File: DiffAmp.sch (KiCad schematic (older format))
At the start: 34 parts, among them J1 USB_OTG, J2 Screw_Terminal_1x03, J3 Conn_01x02, J4 Conn_01x02, J5 Conn_01x02, U1 SF_IHXXXXS, U2 TPS7A49, U3 TPS7A30, U4 OPA189

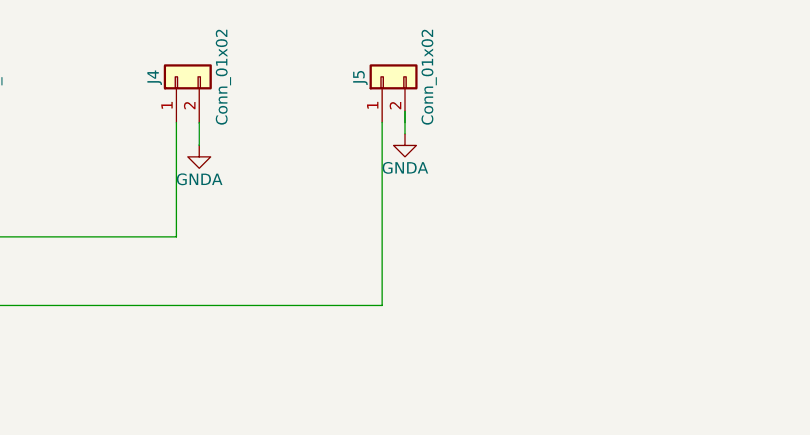
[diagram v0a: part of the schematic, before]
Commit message: Begin Layouting
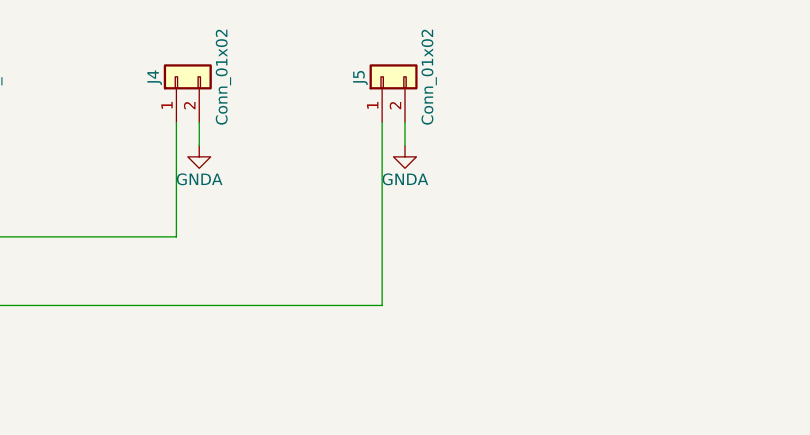
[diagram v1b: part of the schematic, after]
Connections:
- net GNDA: now also J5.2 (Pin_2)
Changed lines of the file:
@@
 L GNDA #PWR08
 U 1 1 5AA11818
-P 6300 1350
-F 0 "#PWR08" H 6300 1100 50  0001 C CNN
-F 1 "GNDA" H 6300 1200 50  0000 C CNN
-F 2 "" H 6300 1350 50  0001 C CNN
-F 3 "" H 6300 1350 50  0001 C CNN
-	1    6300 1350
+P 6300 1400
+F 0 "#PWR08" H 6300 1150 50  0001 C CNN
+F 1 "GNDA" H 6300 1250 50  0000 C CNN
+F 2 "" H 6300 1400 50  0001 C CNN
+F 3 "" H 6300 1400 50  0001 C CNN
+	1    6300 1400
 	1    0    0    -1
 $EndComp
@@
 	900  1900 1050 1900
 Wire Wire Line
-	6300 1250 6300 1350
+	6300 1300 6300 1400
 $Comp
 L USB_OTG J1
